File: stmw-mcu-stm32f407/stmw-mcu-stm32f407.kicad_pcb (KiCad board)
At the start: 4 copper layers, 69 x 43.5 mm, 41 parts, among them J2 TYPE-C-31-M-12, SW1 TS-1088R-02526, SW2 TS-1088R-02526, U1 AMS1117-3.3, U3 STM32F407VETx, Y1 X_16MHZ

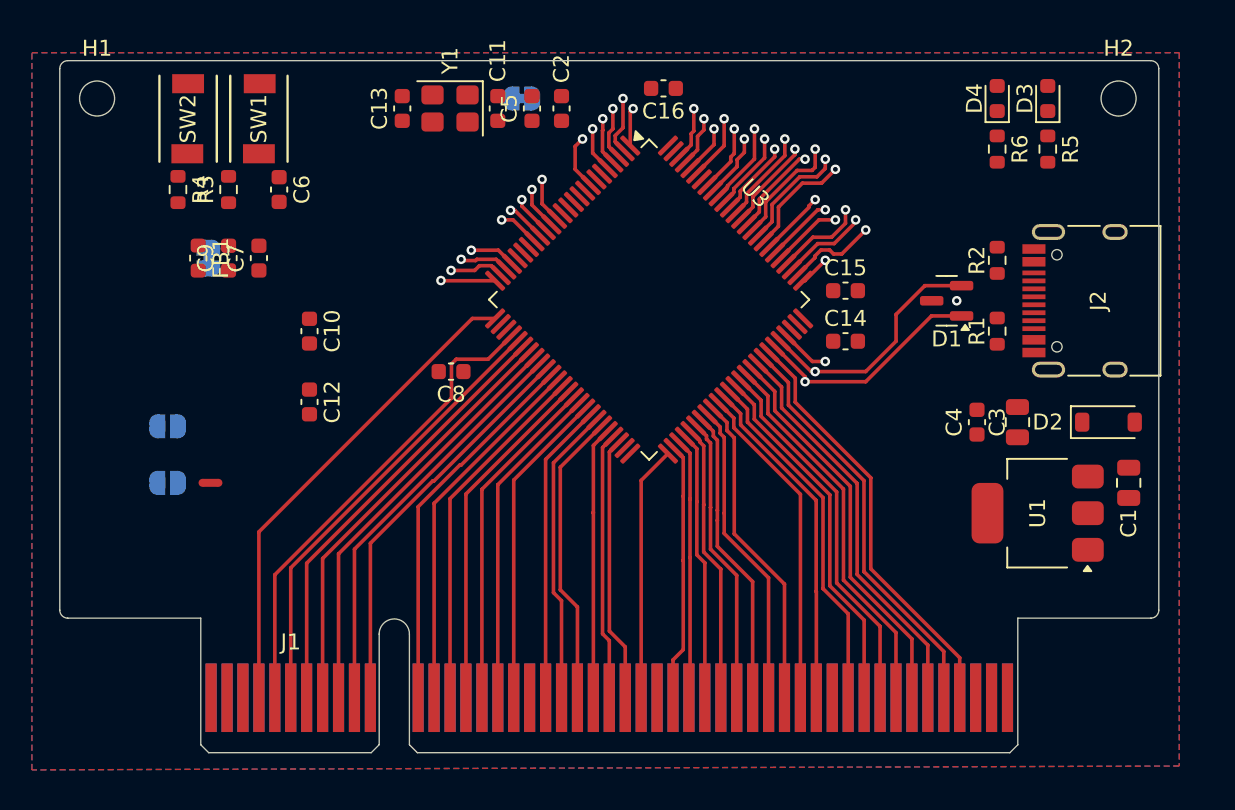
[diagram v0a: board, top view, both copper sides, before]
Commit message: Hmmm
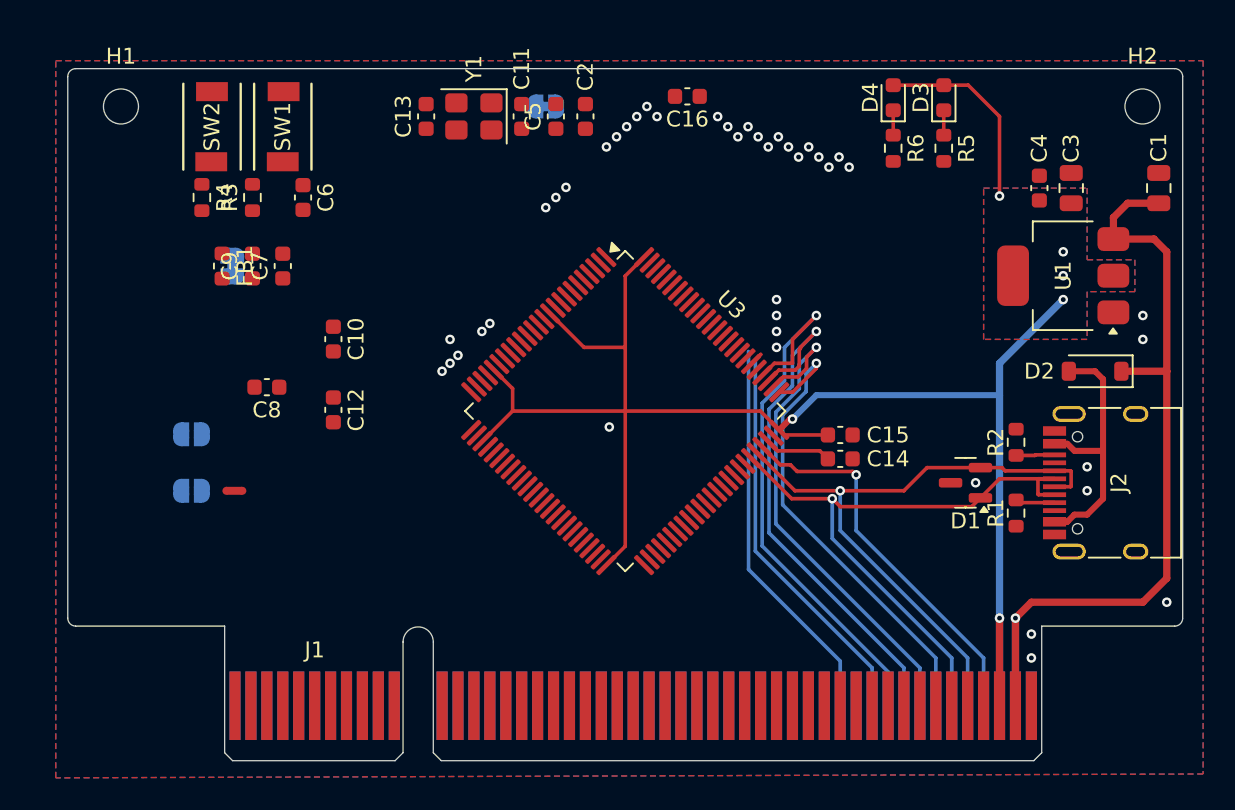
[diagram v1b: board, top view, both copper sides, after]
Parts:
- C1, C3: value C_10UF_0805 -> 10uF
- C10, C15, C16, C2, C5, C6, C7, C8, C9: value C_100NF_0603 -> 100nF
- C11, C13: value C_20PF_0603 -> 20pF
- C4: value C_1UF_0603 -> 1uF
- moved C1 18.6 mm to (183.5, 85.0), turned to 90 degrees
- moved C4 15.2 mm to (176.0, 85.0)
- moved C3 15.1 mm to (178.0, 85.0)
- moved U1 15.0 mm to (177.5, 90.5)
- moved C8 11.6 mm to (127.5, 97.5)
- moved J2 11.5 mm to (181.0, 103.5)
- moved D1 11.5 mm to (171.4, 103.5)
- moved R1 11.5 mm to (174.5, 105.4)
- moved R2 11.5 mm to (174.5, 101.0)
- moved C15 9.07 mm to (163.5, 100.5)
- moved C14 7.39 mm to (163.5, 102.0)
- moved U3 7.16 mm to (150.0, 99.0)
- moved D3 6.53 mm to (170.0, 79.3)
- moved D4 6.53 mm to (166.8, 79.3)
- moved R5 6.53 mm to (170.0, 82.5)
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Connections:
- J1 pad A20: PE1 -> (no net)
- J1 pad A26: PB5 -> (no net)
- J1 pad A28: PB4 -> (no net)
- U3 pad 21: unconnected-(U3-VREF+-Pad21) -> +3V3
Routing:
- net +3V3: track 0.00 -> 112.0 mm, vias 0 -> 6
- net +5V: track 0.00 -> 53.1 mm, vias 0 -> 1
- net PA3: track 30.8 -> 0.00 mm
- net PA4: track 30.1 -> 0.00 mm
- net PC11: track 5.63 -> 35.0 mm
- net PA5: track 28.3 -> 0.00 mm
- net PC10: track 5.38 -> 33.2 mm
- net PA14: track 1.92 -> 29.6 mm
- net PA6: track 27.7 -> 0.00 mm
- net PA7: track 27.1 -> 0.00 mm
- net PA10: track 26.6 -> 0.00 mm
- net PC4: track 26.4 -> 0.00 mm
- net PA9: track 26.0 -> 0.00 mm
- net PC5: track 25.8 -> 0.00 mm
- net PA15: track 5.72 -> 31.4 mm
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- added copper zone on B.Cu, net +3V3
- added copper zone on F.Cu, net +3V3
- removed copper zone on In1.Cu, net +3V3
- removed copper zone on In2.Cu, net GND
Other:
- board size 69 x 43.5 mm -> 70 x 43.5 mm
- copper layers 4 -> 2
